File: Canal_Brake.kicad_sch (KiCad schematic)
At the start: 0 parts

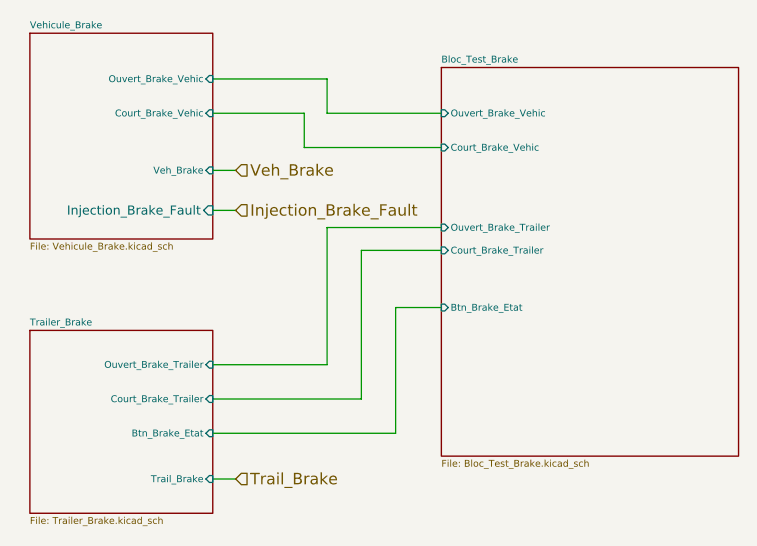
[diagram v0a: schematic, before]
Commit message: Add files via upload
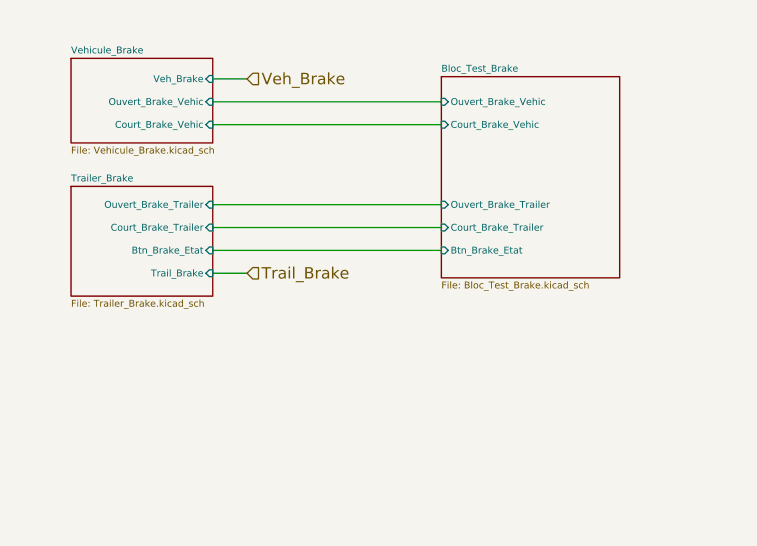
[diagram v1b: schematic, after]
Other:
- sheet Vehicule_Brake ports: added none; removed Injection_Brake_Fault
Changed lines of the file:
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@@
 	(wire
 		(pts
-			(xy 48.26 29.21) (xy 48.26 33.02)
-		)
-		(stroke
-			(width 0)
-			(type default)
-		)
-	)
-	(wire
-		(pts
-			(xy 58.42 64.77) (xy 58.42 50.8)
-		)
-		(stroke
-			(width 0)
-			(type default)
-		)
-	)
-	(wire
-		(pts
-			(xy 50.8 25.4) (xy 50.8 29.21)
-		)
-		(stroke
-			(width 0)
-			(type default)
-		)
-	)
-	(wire
-		(pts
-			(xy 38.1 57.15) (xy 50.8 57.15)
-		)
-		(stroke
-			(width 0)
-			(type default)
-		)
-	)
-	(wire
-		(pts
-			(xy 58.42 50.8) (xy 63.5 50.8)
-		)
-		(stroke
-			(width 0)
-			(type default)
-		)
-	)
-	(wire
-		(pts
-			(xy 50.8 29.21) (xy 63.5 29.21)
-		)
-		(stroke
-			(width 0)
-			(type default)
-		)
-	)
-	(wire
-		(pts
-			(xy 54.61 44.45) (xy 63.5 44.45)
-		)
-		(stroke
-			(width 0)
-			(type default)
-		)
-	)
-	(wire
-		(pts
-			(xy 38.1 60.96) (xy 54.61 60.96)
-		)
-		(stroke
-			(width 0)
-			(type default)
-		)
-	)
-	(wire
-		(pts
-			(xy 48.26 33.02) (xy 63.5 33.02)
-		)
-		(stroke
-			(width 0)
-			(type default)
-		)
-	)
-	(wire
-		(pts
-			(xy 38.1 64.77) (xy 58.42 64.77)
-		)
-		(stroke
-			(width 0)
-			(type default)
-		)
-	)
-	(wire
-		(pts
-			(xy 54.61 60.96) (xy 54.61 44.45)
-		)
-		(stroke
-			(width 0)
-			(type default)
-		)
-	)
-	(wire
-		(pts
-			(xy 50.8 41.91) (xy 63.5 41.91)
-		)
-		(stroke
-			(width 0)
-			(type default)
-		)
-	)
-	(wire
-		(pts
-			(xy 38.1 29.21) (xy 48.26 29.21)
-		)
-		(stroke
-			(width 0)
-			(type default)
-		)
-	)
-	(wire
-		(pts
-			(xy 38.1 69.85) (xy 40.64 69.85)
-		)
-		(stroke
-			(width 0)
-			(type default)
-		)
-	)
-	(wire
-		(pts
-			(xy 38.1 40.005) (xy 40.64 40.005)
-		)
-		(stroke
-			(width 0)
-			(type default)
-		)
-	)
-	(wire
-		(pts
-			(xy 38.1 35.56) (xy 40.64 35.56)
-		)
-		(stroke
-			(width 0)
-			(type default)
-		)
-	)
-	(wire
-		(pts
-			(xy 38.1 25.4) (xy 50.8 25.4)
-		)
-		(stroke
-			(width 0)
-			(type default)
-		)
-	)
-	(wire
-		(pts
-			(xy 50.8 57.15) (xy 50.8 41.91)
-		)
-		(stroke
-			(width 0)
-			(type default)
-		)
-	)
-	(hierarchical_label "Injection_Brake_Fault"
+			(xy 38.1 39.37) (xy 63.5 39.37)
+		)
+		(stroke
+			(width 0)
+			(type default)
+		)
+	)
+	(wire
+		(pts
+			(xy 38.1 41.91) (xy 63.5 41.91)
+		)
+		(stroke
+			(width 0)
+			(type default)
+		)
+	)
+	(wire
+		(pts
+			(xy 38.1 44.45) (xy 63.5 44.45)
+		)
+		(stroke
+			(width 0)
+			(type default)
+		)
+	)
+	(wire
+		(pts
+			(xy 38.1 30.48) (xy 63.5 30.48)
+		)
+		(stroke
+			(width 0)
+			(type default)
+		)
+	)
+	(wire
+		(pts
+			(xy 38.1 46.99) (xy 41.91 46.99)
+		)
+		(stroke
+			(width 0)
+			(type default)
+		)
+	)
+	(wire
+		(pts
+			(xy 38.1 25.4) (xy 41.91 25.4)
+		)
+		(stroke
+			(width 0)
+			(type default)
+		)
+	)
+	(wire
+		(pts
+			(xy 38.1 27.94) (xy 63.5 27.94)
+		)
+		(stroke
+			(width 0)
+			(type default)
+		)
+	)
+	(hierarchical_label "Trail_Brake"
 		(shape input)
-		(at 40.64 40.005 0)
+		(at 41.91 46.99 0)
 		(effects
 			(font
@@
 		)
 	)
-	(hierarchical_label "Trail_Brake"
+	(hierarchical_label "Veh_Brake"
 		(shape input)
-		(at 40.64 69.85 0)
+		(at 41.91 25.4 0)
 		(effects
 			(font
@@
 		)
 	)
-	(hierarchical_label "Veh_Brake"
-		(shape input)
-		(at 40.64 35.56 0)
-		(effects
-			(font
-				(size 1.27 1.27)
-			)
-			(justify left)
-		)
-	)
 	(sheet
-		(at 17.78 20.32)
-		(size 20.32 22.86)
+		(at 22.352 23.114)
+		(size 15.748 9.398)
 		(exclude_from_sim no)
 		(in_bom yes)
@@
 		)
 		(property "Sheetname" "Vehicule_Brake"
-			(at 17.78 19.8624 0)
+			(at 22.352 22.6564 0)
 			(show_name no)
 			(do_not_autoplace no)
@@
 		)
 		(property "Sheetfile" "Vehicule_Brake.kicad_sch"
-			(at 17.78 43.5614 0)
+			(at 22.352 32.8934 0)
 			(show_name no)
 			(do_not_autoplace no)
@@
 		)
 		(pin "Ouvert_Brake_Vehic" input
+			(at 38.1 27.94 0)
+			(effects
+				(font
+					(size 0.762 0.762)
+				)
+				(justify right)
+			)
+		)
+		(pin "Court_Brake_Vehic" input
+			(at 38.1 30.48 0)
+			(effects
+				(font
+					(size 0.762 0.762)
+				)
+				(justify right)
+			)
+		)
+		(pin "Veh_Brake" input
 			(at 38.1 25.4 0)
 			(effects
 				(font
 					(size 0.762 0.762)
-				)
-				(justify right)
-			)
-		)
-		(pin "Court_Brake_Vehic" input
-			(at 38.1 29.21 0)
-			(effects
-				(font
-					(size 0.762 0.762)
-				)
-				(justify right)
-			)
-		)
-		(pin "Veh_Brake" input
-			(at 38.1 35.56 0)
-			(effects
-				(font
-					(size 0.762 0.762)
-				)
-				(justify right)
-			)
-		)
-		(pin "Injection_Brake_Fault" input
-			(at 38.1 40.005 0)
-			(effects
-				(font
-					(size 1.016 1.016)
 				)
 				(justify right)
@@
 	)
 	(sheet
-		(at 17.78 53.34)
-		(size 20.32 20.32)
+		(at 22.352 37.338)
+		(size 15.748 12.192)
 		(exclude_from_sim no)
 		(in_bom yes)
@@
 		)
 		(property "Sheetname" "Trailer_Brake"
-			(at 17.78 52.8824 0)
+			(at 22.352 36.8804 0)
 			(show_name no)
 			(do_not_autoplace no)
@@
 		)
 		(property "Sheetfile" "Trailer_Brake.kicad_sch"
-			(at 17.78 74.0414 0)
+			(at 22.352 49.9114 0)
 			(show_name no)
 			(do_not_autoplace no)
@@
 		)
 		(pin "Trail_Brake" input
-			(at 38.1 69.85 0)
+			(at 38.1 46.99 0)
 			(effects
 				(font
@@
 		)
 		(pin "Ouvert_Brake_Trailer" input
-			(at 38.1 57.15 0)
+			(at 38.1 39.37 0)
 			(effects
 				(font
@@
 		)
 		(pin "Btn_Brake_Etat" input
-			(at 38.1 64.77 0)
+			(at 38.1 44.45 0)
 			(effects
 				(font
@@
 		)
 		(pin "Court_Brake_Trailer" input
-			(at 38.1 60.96 0)
+			(at 38.1 41.91 0)
 			(effects
 				(font
@@
 	)
 	(sheet
-		(at 63.5 24.13)
-		(size 33.02 43.18)
+		(at 63.5 25.146)
+		(size 19.812 22.352)
 		(exclude_from_sim no)
 		(in_bom yes)
@@
 		)
 		(property "Sheetname" "Bloc_Test_Brake"
-			(at 63.5 23.6724 0)
+			(at 63.5 24.6884 0)
 			(show_name no)
 			(do_not_autoplace no)
@@
 		)
 		(property "Sheetfile" "Bloc_Test_Brake.kicad_sch"
-			(at 63.5 67.6914 0)
+			(at 63.5 47.8794 0)
 			(show_name no)
 			(do_not_autoplace no)
@@
 		)
 		(pin "Ouvert_Brake_Trailer" input
+			(at 63.5 39.37 180)
+			(effects
+				(font
+					(size 0.762 0.762)
+				)
+				(justify left)
+			)
+		)
+		(pin "Ouvert_Brake_Vehic" input
+			(at 63.5 27.94 180)
+			(effects
+				(font
+					(size 0.762 0.762)
+				)
+				(justify left)
+			)
+		)
+		(pin "Btn_Brake_Etat" input
+			(at 63.5 44.45 180)
+			(effects
+				(font
+					(size 0.762 0.762)
+				)
+				(justify left)
+			)
+		)
+		(pin "Court_Brake_Trailer" input
 			(at 63.5 41.91 180)
 			(effects
@@
 			)
 		)
-		(pin "Ouvert_Brake_Vehic" input
-			(at 63.5 29.21 180)
-			(effects
-				(font
-					(size 0.762 0.762)
-				)
-				(justify left)
-			)
-		)
-		(pin "Btn_Brake_Etat" input
-			(at 63.5 50.8 180)
-			(effects
-				(font
-					(size 0.762 0.762)
-				)
-				(justify left)
-			)
-		)
-		(pin "Court_Brake_Trailer" input
-			(at 63.5 44.45 180)
-			(effects
-				(font
-					(size 0.762 0.762)
-				)
-				(justify left)
-			)
-		)
 		(pin "Court_Brake_Vehic" input
-			(at 63.5 33.02 180)
-			(effects
-				(font
+			(at 63.5 30.48 180)
+			(effects
+				(font
